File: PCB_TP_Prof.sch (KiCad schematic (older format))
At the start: 8 parts, among them J1 Conn_01x04_Female, J2 Conn_01x01_Male

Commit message: update files
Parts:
- removed J1: Conn_01x04_Female, Connector_PinHeader_2.54mm:PinHeader_1x04_P2.54mm_Vertical, symbol Connector:Conn_01x04_Female
- removed J2: Conn_01x01_Male, Connector_PinHeader_2.54mm:PinHeader_1x01_P2.54mm_Vertical, symbol Connector:Conn_01x01_Male
- added J2: Conn_01x12_Female, Connector_PinHeader_2.54mm:PinHeader_1x12_P2.54mm_Vertical, symbol Connector:Conn_01x12_Female
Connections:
- wire segments 34 -> 68
- no-connect marks 0 -> 1
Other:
- note added: "DT y SCK pueden ir a \ncualquier GPIO de la EDU-CIAA"
- note added: "LL\n"
- note added: "LR"
- note added: "UL\n"
- note added: "UR\n"
- moved on the sheet: JP1, R4, U_MUX1

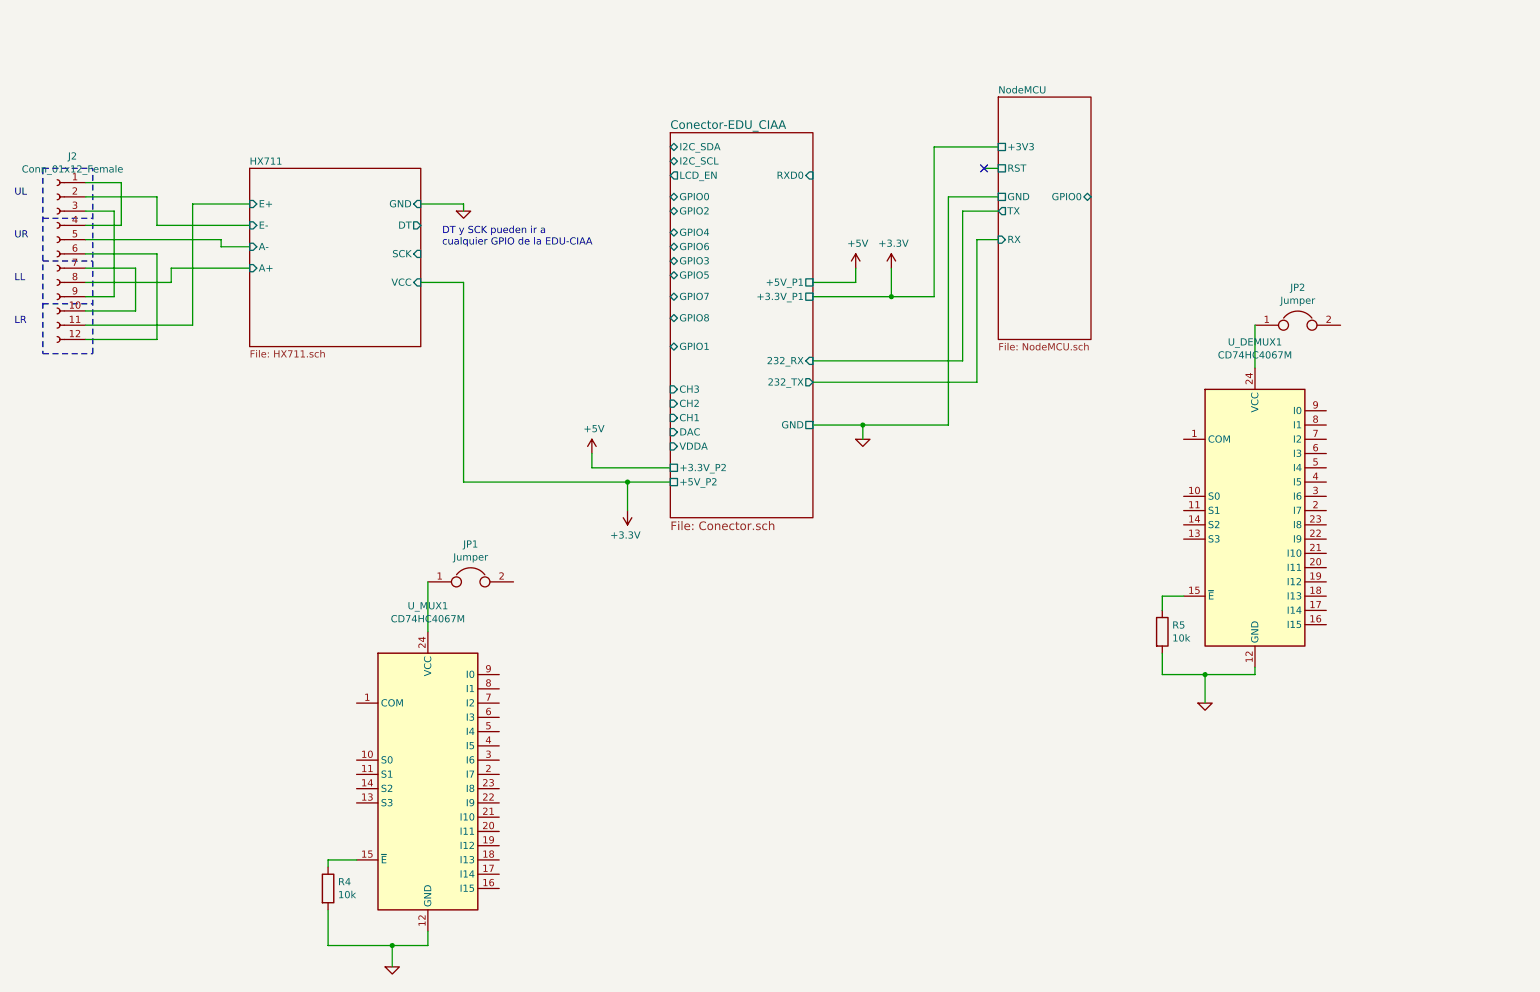
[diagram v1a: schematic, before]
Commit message: update files
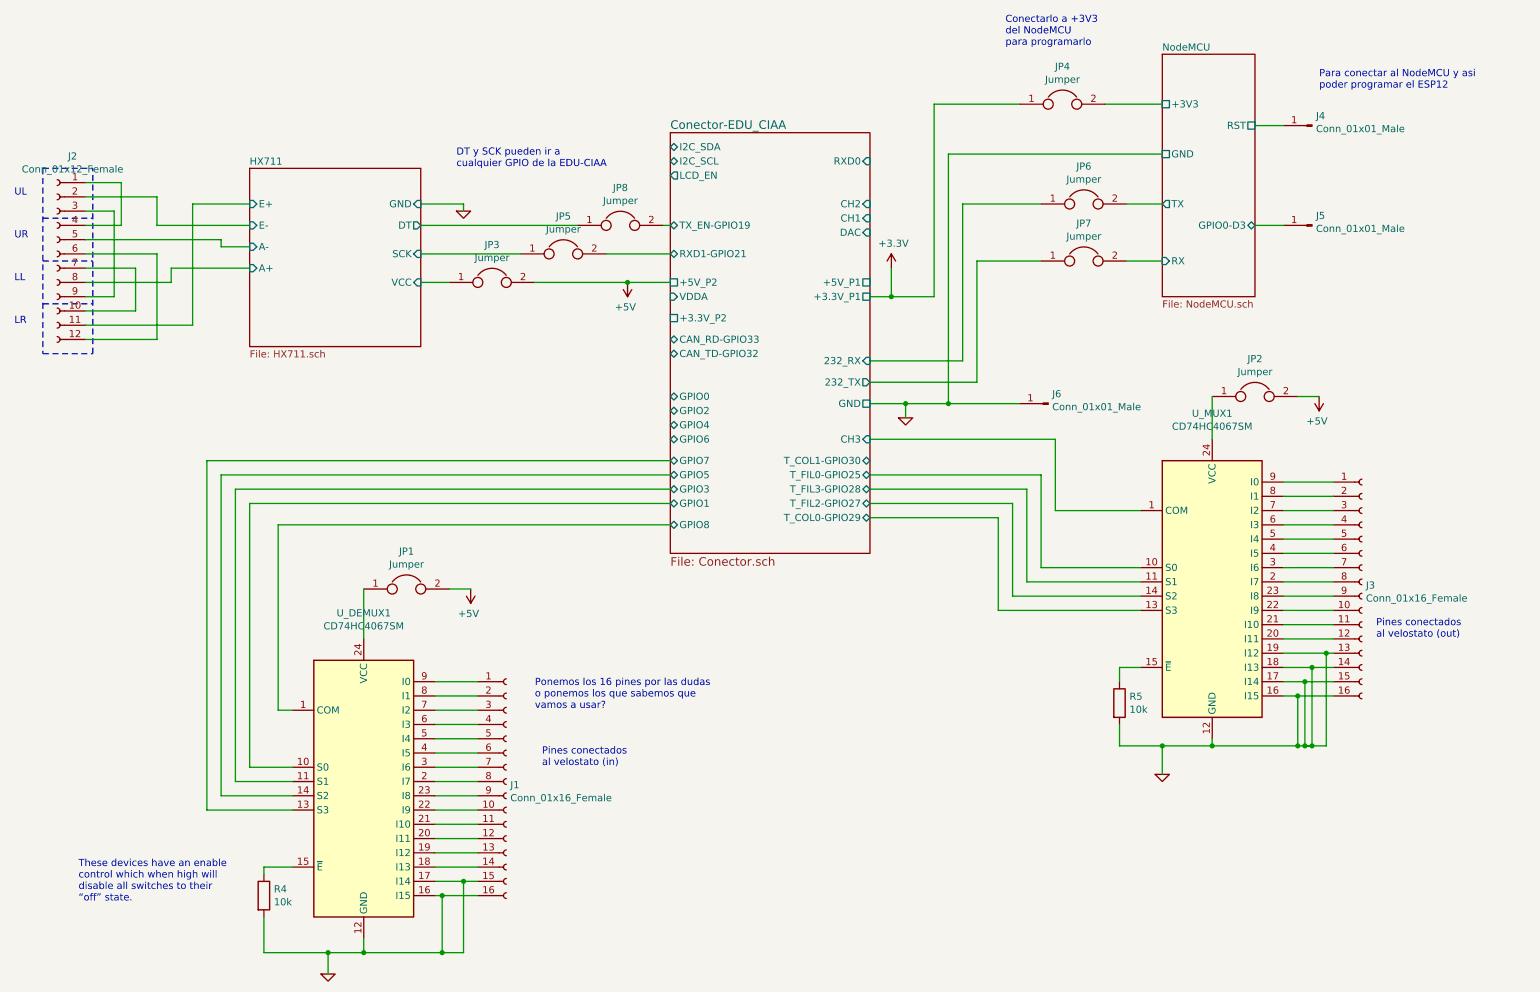
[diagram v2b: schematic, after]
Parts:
- removed U_DEMUX1, U_MUX1: CD74HC4067M, Package_SO:SOIC-24W_7.5x15.4mm_P1.27mm, symbol 74xx:CD74HC4067M
- added J1, J3: Conn_01x16_Female, Connector_PinHeader_2.54mm:PinHeader_1x16_P2.54mm_Vertical, symbol Connector:Conn_01x16_Female
- added J4, J5, J6: Conn_01x01_Male, Connector_PinHeader_2.54mm:PinHeader_1x01_P2.54mm_Vertical, symbol Connector:Conn_01x01_Male
- added JP3, JP4, JP5, JP6, JP7, JP8: Jumper, Connector_PinHeader_2.54mm:PinHeader_1x02_P2.54mm_Vertical, symbol Device:Jumper
- added U_DEMUX1, U_MUX1: CD74HC4067SM, Package_SO:SSOP-24_5.3x8.2mm_P0.65mm, symbol 74xx:CD74HC4067SM
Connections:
- net +3V3: now also JP4.1
- net +5V: now also JP1.2, JP2.2, JP3.2
- net Conector-EDU_CIAA/232_RX: now also JP6.1
- net Conector-EDU_CIAA/232_TX: now also JP7.1
- net Conector-EDU_CIAA/CH3: now also U_MUX1.1 (COM)
- net Conector-EDU_CIAA/GPIO1: now also U_DEMUX1.10 (S0)
- net Conector-EDU_CIAA/GPIO3: now also U_DEMUX1.11 (S1)
- net Conector-EDU_CIAA/GPIO5: now also U_DEMUX1.14 (S2)
- net Conector-EDU_CIAA/GPIO7: now also U_DEMUX1.13 (S3)
- net Conector-EDU_CIAA/GPIO8: now also U_DEMUX1.1 (COM)
- net GND: now also J1.15 (Pin_15), J1.16 (Pin_16), J3.13 (Pin_13), J3.14 (Pin_14), J3.15 (Pin_15), J3.16 (Pin_16), J6.1 (Pin_1), U_DEMUX1.12 (GND), U_DEMUX1.16 (I15), U_DEMUX1.17 (I14), U_MUX1.12 (GND), U_MUX1.16 (I15), U_MUX1.17 (I14), U_MUX1.18 (I13), U_MUX1.19 (I12)
- net HX711/DT: now also JP8.1
- net HX711/SCK: now also JP5.1
- net NodeMCU/RST: now also J4.1 (Pin_1)
- net at R4.1: now also U_DEMUX1.15 (~E)
- net at JP1.1: now also U_DEMUX1.24 (VCC)
- net at R5.1: now also U_MUX1.15 (~E)
- net at JP2.1: now also U_MUX1.24 (VCC)
- new net: J1.1 (Pin_1), U_DEMUX1.9 (I0)
- new net: J1.10 (Pin_10), U_DEMUX1.22 (I9)
- new net: J1.11 (Pin_11), U_DEMUX1.21 (I10)
- new net: J1.12 (Pin_12), U_DEMUX1.20 (I11)
- new net: J1.13 (Pin_13), U_DEMUX1.19 (I12)
- new net: J1.14 (Pin_14), U_DEMUX1.18 (I13)
- new net: J1.2 (Pin_2), U_DEMUX1.8 (I1)
- new net: J1.3 (Pin_3), U_DEMUX1.7 (I2)
- new net: J1.4 (Pin_4), U_DEMUX1.6 (I3)
- new net: J1.5 (Pin_5), U_DEMUX1.5 (I4)
- new net: J1.6 (Pin_6), U_DEMUX1.4 (I5)
- new net: J1.7 (Pin_7), U_DEMUX1.3 (I6)
- new net: J1.8 (Pin_8), U_DEMUX1.2 (I7)
- new net: J1.9 (Pin_9), U_DEMUX1.23 (I8)
- new net: J3.1 (Pin_1), U_MUX1.9 (I0)
- new net: J3.10 (Pin_10), U_MUX1.22 (I9)
- new net: J3.11 (Pin_11), U_MUX1.21 (I10)
- new net: J3.12 (Pin_12), U_MUX1.20 (I11)
- new net: J3.2 (Pin_2), U_MUX1.8 (I1)
- new net: J3.3 (Pin_3), U_MUX1.7 (I2)
- new net: J3.4 (Pin_4), U_MUX1.6 (I3)
- new net: J3.5 (Pin_5), U_MUX1.5 (I4)
- new net: J3.6 (Pin_6), U_MUX1.4 (I5)
- new net: J3.7 (Pin_7), U_MUX1.3 (I6)
- new net: J3.8 (Pin_8), U_MUX1.2 (I7)
- new net: J3.9 (Pin_9), U_MUX1.23 (I8)
- new net Conector-EDU_CIAA/RXD1-GPIO21: JP5.2
- new net Conector-EDU_CIAA/TX_EN-GPIO19: JP8.2
- new net Conector-EDU_CIAA/T_COL0-GPIO29: U_MUX1.13 (S3)
- new net Conector-EDU_CIAA/T_FIL0-GPIO25: U_MUX1.10 (S0)
- new net Conector-EDU_CIAA/T_FIL2-GPIO27: U_MUX1.14 (S2)
- new net Conector-EDU_CIAA/T_FIL3-GPIO28: U_MUX1.11 (S1)
- new net HX711/VCC: JP3.1
- new net NodeMCU/+3V3: JP4.2
- new net NodeMCU/GPIO0-D3: J5.1 (Pin_1)
- new net NodeMCU/RX: JP7.2
- new net NodeMCU/TX: JP6.2
- no-connect marks 1 -> 0
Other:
- note added: "Conectarlo a +3V3\ndel NodeMCU \npara programarlo"
- note added: "Para conectar al NodeMCU y asi \npoder programar el ESP12\n"
- note added: "Pines conectados \nal velostato (in)\n"
- note added: "Pines conectados \nal velostato (out)\n"
- note added: "Ponemos los 16 pines por las dudas\no ponemos los que sabemos que \nvamos a usar?\n"
- note added: "These devices have an enable \ncontrol which when high will \ndisable all switches to their \n“off” state."
- moved on the sheet: JP1, JP2, R4, R5

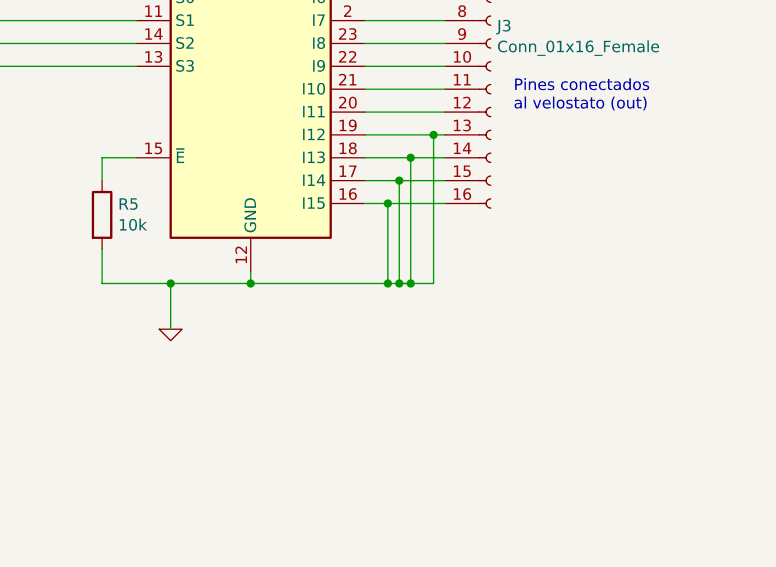
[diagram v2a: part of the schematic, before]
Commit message: Update files
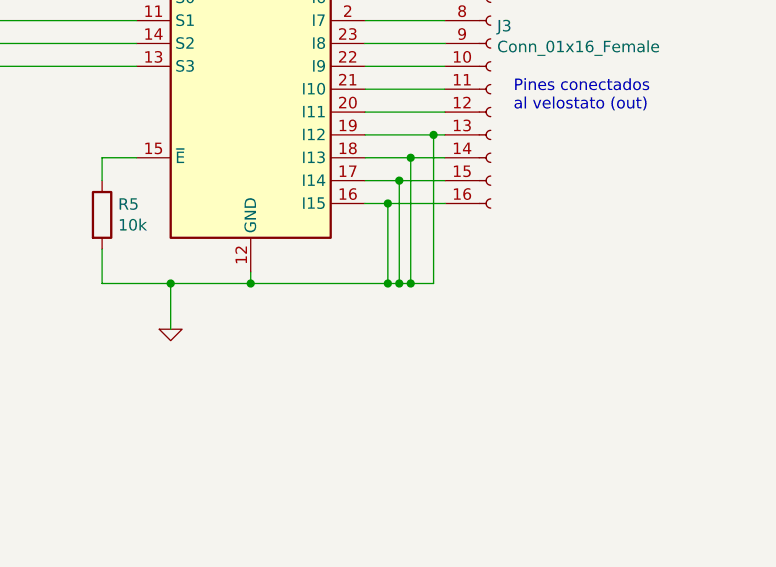
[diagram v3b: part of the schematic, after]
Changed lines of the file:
@@
 	10000 5250 9700 5250
 Connection ~ 9900 5900
-Wire Wire Line
-	9900 5900 9850 5900
 $EndSCHEMATC
